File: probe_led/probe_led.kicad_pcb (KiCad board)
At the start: 2 copper layers, 60.2 x 68.5 mm, 14 parts, among them U1 IRM-H638T_TR2, U2 IRM-H638T_TR2, U3 IRM-H638T_TR2

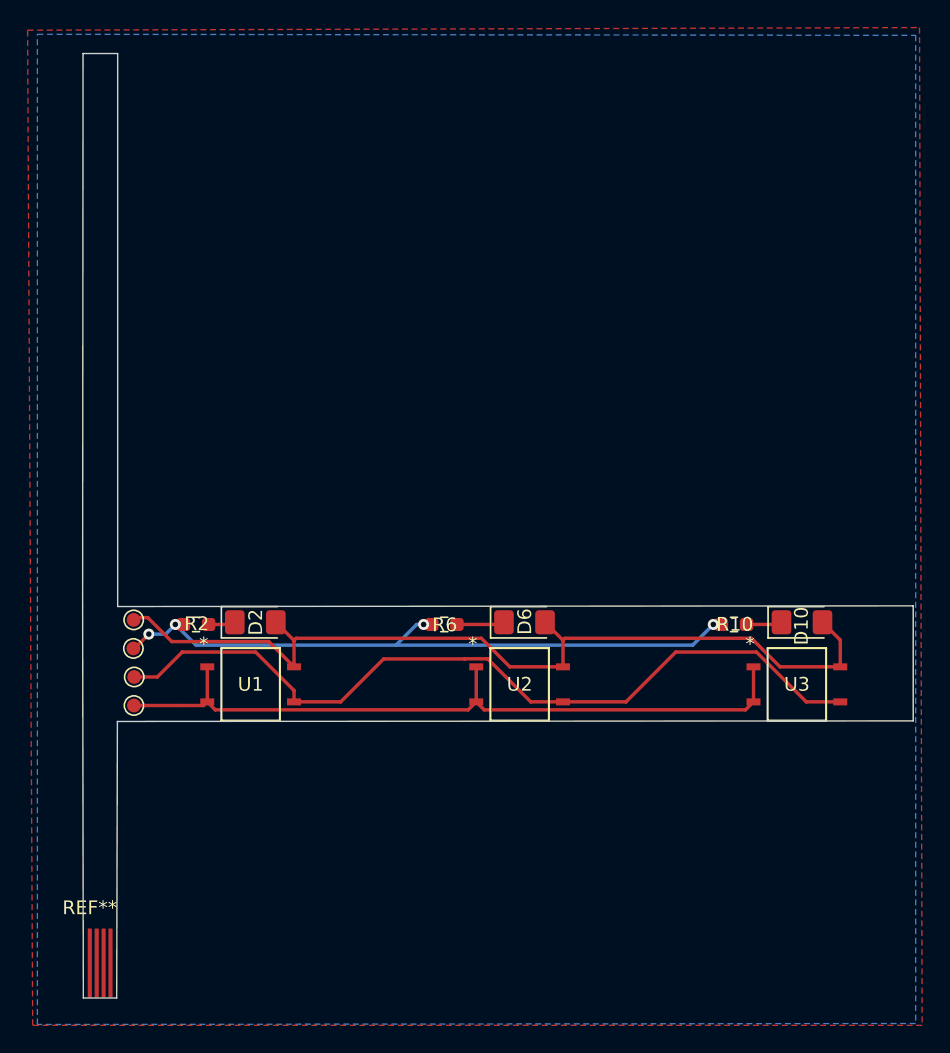
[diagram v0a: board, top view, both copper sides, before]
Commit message: -prepare for production
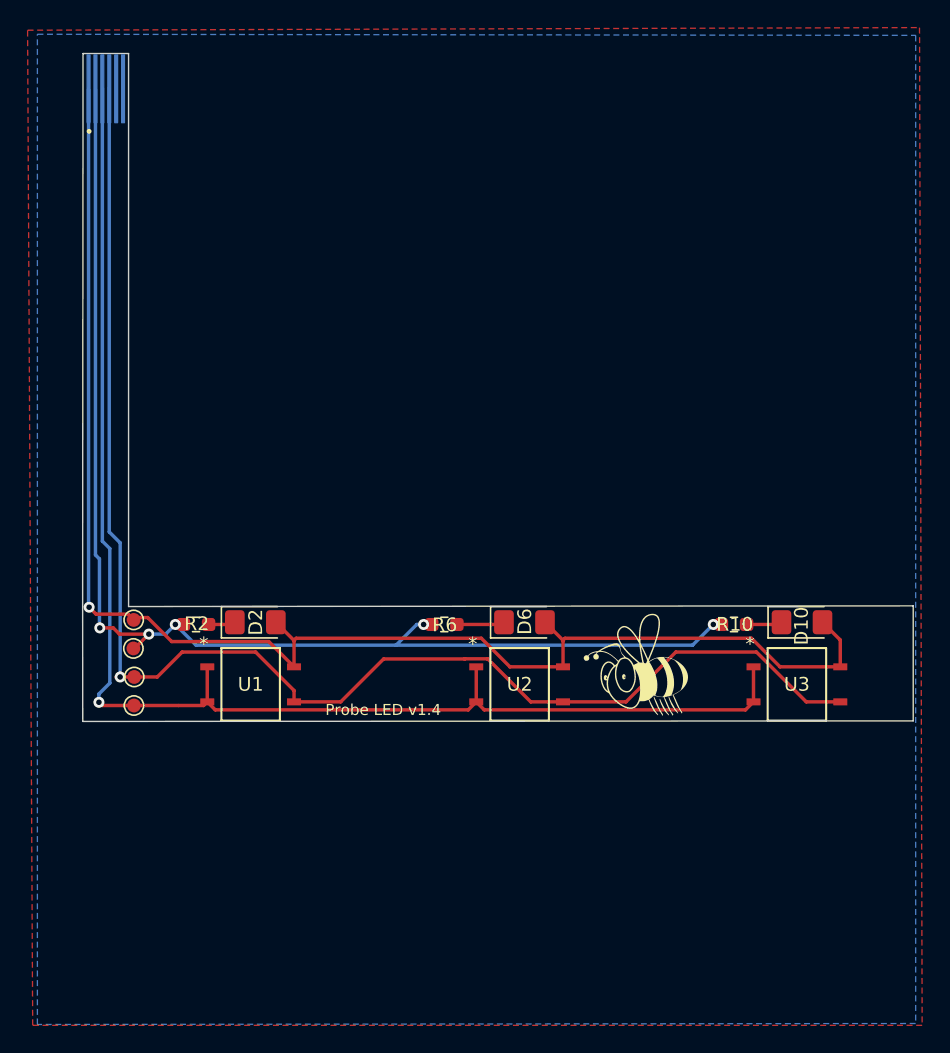
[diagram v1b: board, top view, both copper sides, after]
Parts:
- removed REF**: FPC_4pin_0.5mm_fingers, Connector_FFC-FPC:FPC_4pin_0.5mm_fingers
- added  : Probe LED v1.4, LOGO, F.Cu at (138.0, 81.0)
- added J3: Conn_01x06, Library:FPC_4pin_0.5mm_fingers, B.Cu at (98.2, 39.2)
- 3V3: renamed from 5V1; value 5V -> 33V
- renumbered LED-1 to IRLED_POW1, IR_D1 to IRREC_DATA1, IR-1 to IRREC_POW1
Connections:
- net Net-(D10-A) renamed +3.3V
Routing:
- net Net-(J3-Pin_3): track 53.6 -> 101.3 mm, vias 0 -> 1
- net Net-(J3-Pin_4): track 59.5 -> 104.0 mm, vias 0 -> 1
- net Net-(J3-Pin_2): track 48.4 -> 91.3 mm, vias 4 -> 5
- net +3.3V: track 65.9 -> 107.1 mm, vias 0 -> 1
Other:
- board size 60.2 x 68.5 mm -> 60.2 x 48.4 mm
